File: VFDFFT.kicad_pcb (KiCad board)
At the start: 2 copper layers, 100 x 50 mm, 271 parts, among them J1 USB_C_Receptacle_USB2.0, J10 Conn_01x02_Pin, J11 Conn_01x02_Male, J14 AudioJack3_Ground, J15 USB_C_Receptacle_USB2.0, J2 BATT, J3 FILAMENT+, J4 VFD_SIG, J5 USB_A, J6 Conn_01x03_Socket, J7 Conn_01x03_Socket, J8 Conn_01x02_Pin, J9 Conn_01x02_Pin, Q1 IRL7486MTRPBF, Q10 AO3400A, Q11 AO3400A, Q12 FS5N10S, Q2 ASDM30DN40E, Q3 ASDM30DN40E, Q4 HSCB2903, Q5 HSCB2903, Q6 AP6800, Q7 FS5N10S, Q8 FS5N10S, Q9 AO3400A, U1 IP2368, U10 TPS61170, U11 TPS61170, U12 W25Q128JVS, U13 TPS62170DSG, U14 LM358, U15 LM324, U16 LM3478, U17 LM2738, U18 ES9023, U19 CH340E, U2 78L05_SOT23, U3 TPS40305, U4 LM3478, U5 LM3478, U6 STM32F446VETx, U7 AP6181, U8 HDC1080, U9 OPT3001DNPR, X1 SX1M32.768KM10F30TNN, X2 12.288MHz, Y1 TAXM26M4ZDBDDT2T, Y2 24M

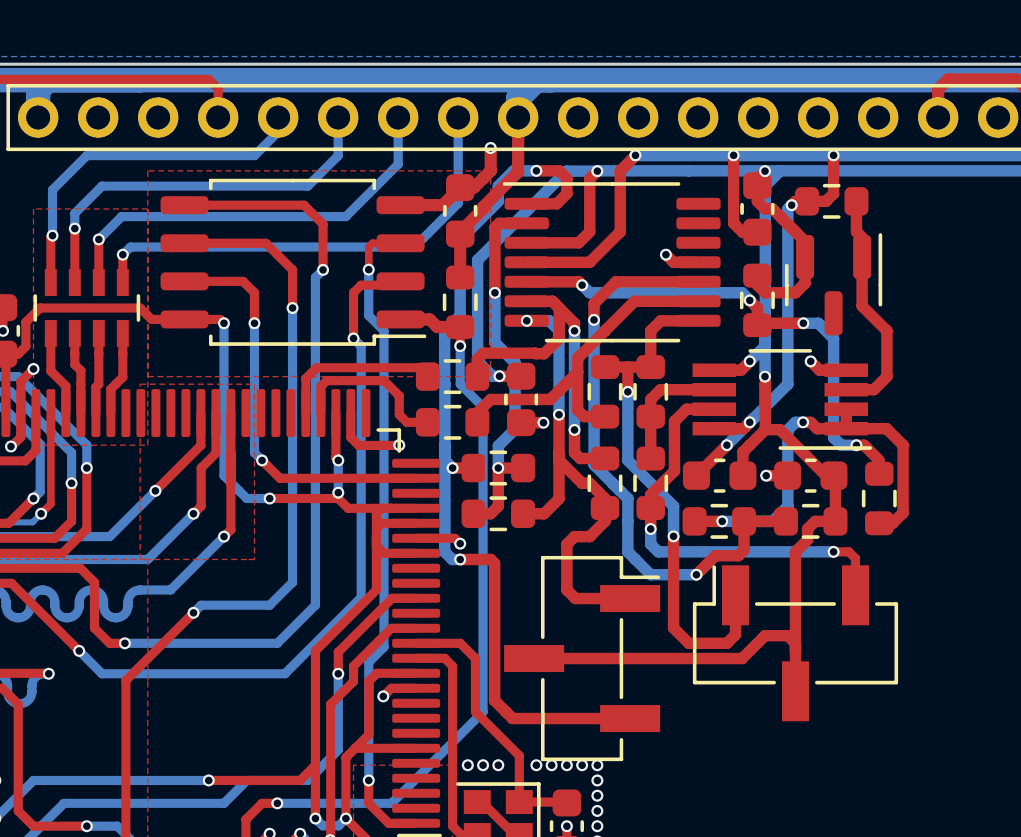
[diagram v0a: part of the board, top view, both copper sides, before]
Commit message: file sync
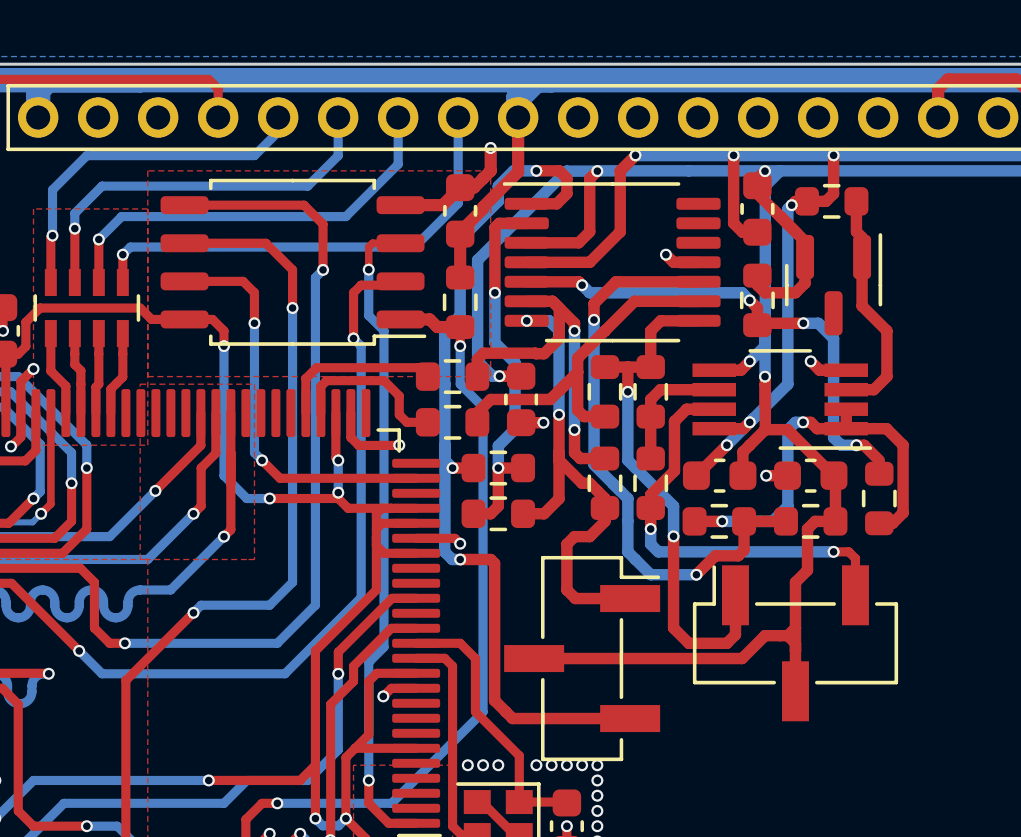
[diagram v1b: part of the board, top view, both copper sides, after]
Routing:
- net GNDA: track 105.7 -> 106.7 mm
